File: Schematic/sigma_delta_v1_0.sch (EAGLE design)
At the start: 32 parts, among them IC1 LM340LZ-05, Q1 BS170, Q2 BS170

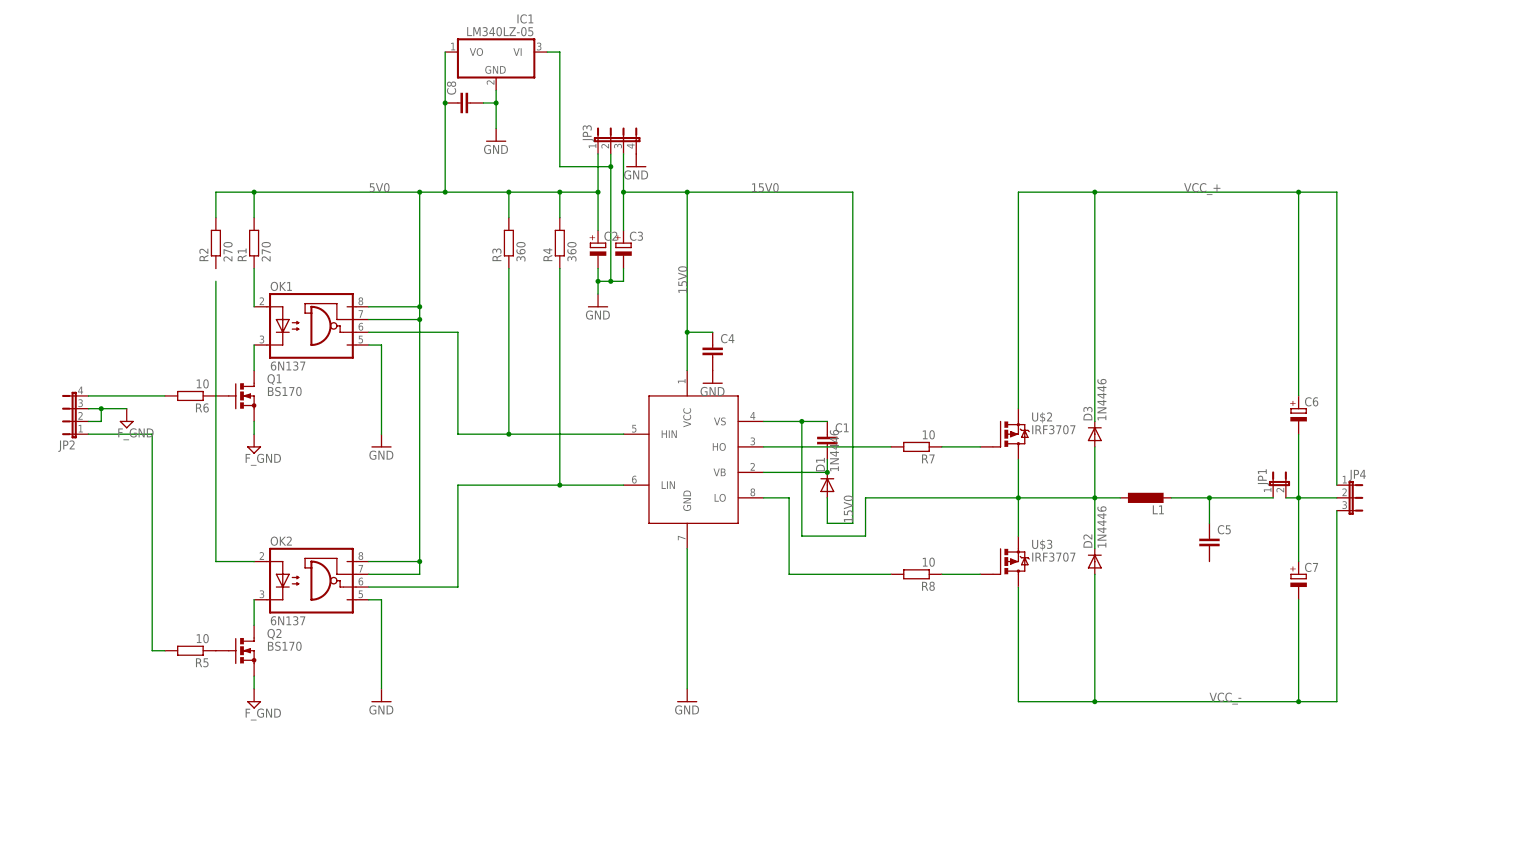
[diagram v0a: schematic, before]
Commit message: started reworking the scematic
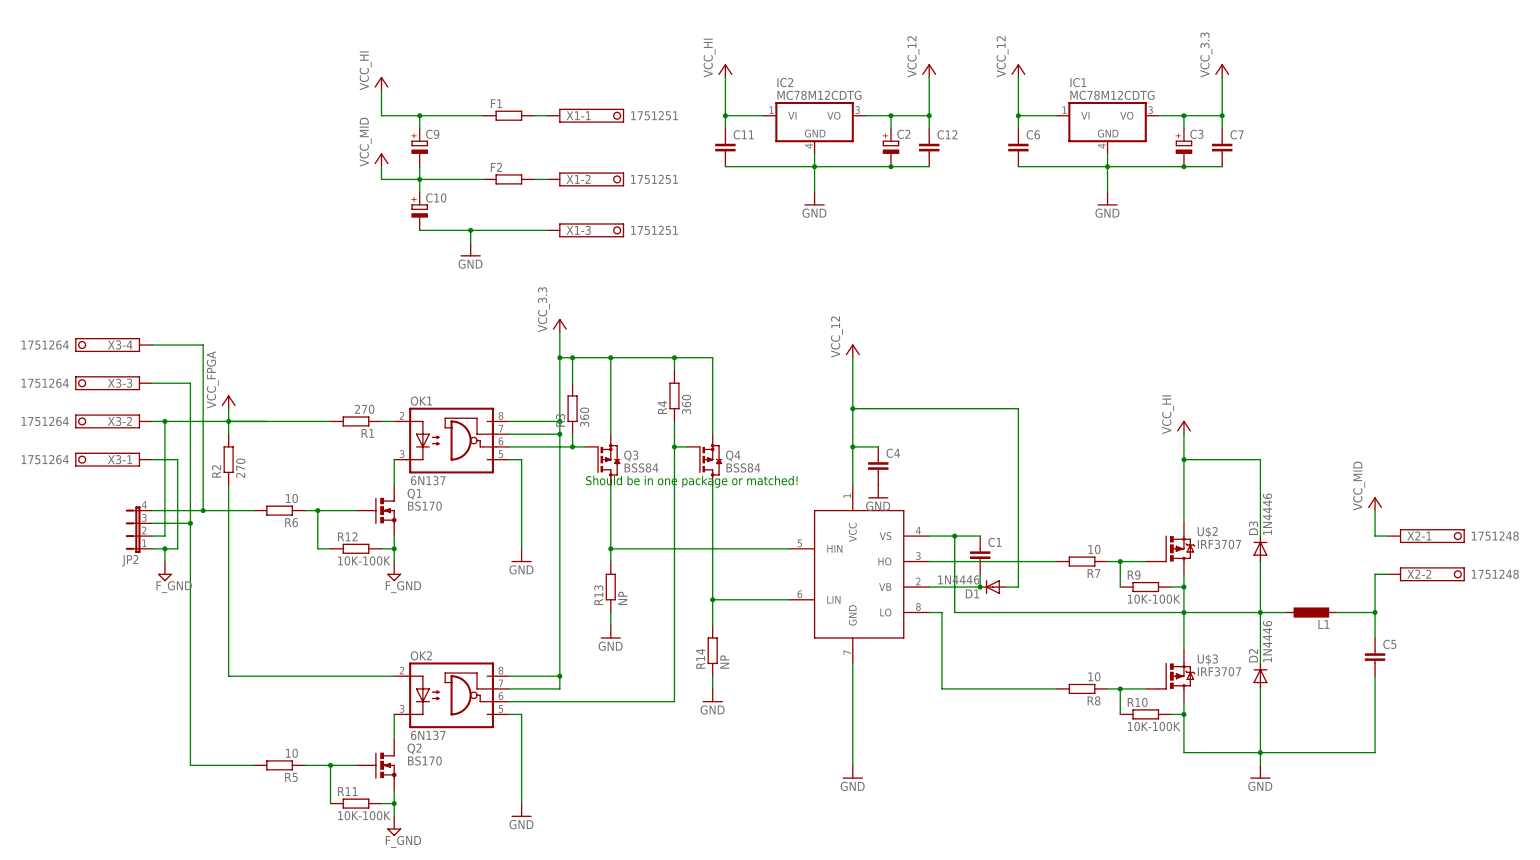
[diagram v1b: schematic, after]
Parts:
- removed C8: (no value), rcl:C-EU025-030X050
- removed JP1: (no value), jumper:JP1E
- removed JP3: (no value), jumper:JP4E
- removed JP4: (no value), jumper:JP2E
- added C10, C9: (no value), rcl:CPOL-EUE2.5-7
- added C11, C12: (no value), rcl:C-EUC0603
- added F1, F2: (no value), rcl:R-EU_M1206
- added IC2: MC78M12CDTG, linear:MC78M12CDTG
- added Q3, Q4: BSS84, transistor-small-signal:BSS84
- added R10, R11, R12, R9: 10K-100K, eagle-ltspice:RR0603
- added R13, R14: NP, eagle-ltspice:RR0603
- added X1: 1751251, con-phoenix-350:1751251
- added X2: 1751248, con-phoenix-350:1751248
- added X3: 1751264, con-phoenix-350:1751264
- C6, C7: device rcl:CPOL-EUE2.5-7 -> rcl:C-EUC0603
- IC1: value LM340LZ-05 -> MC78M12CDTG; device linear:LM340LZ-05 -> linear:MC78M12CDTG
- R1, R2, R3, R4, R5, R6, R7, R8: device eagle-ltspice:R0207/10 -> eagle-ltspice:RR0603
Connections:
- removed net 15V0: C3.+, C4.1, D1.A, JP3.3, U$1.VCC
- removed net 5V0: C2.+, C8.1, IC1.VO, JP3.1, OK1.VCC, OK1.VE, OK2.VCC, OK2.VE, R1.2, R2.2, R3.2, R4.2
- removed net N$8: OK2.VO, R4.1
- removed net VCC_+: C6.+, D3.C, JP4.1, U$2.S
- removed net VCC_-: C7.-, D2.A, JP4.3, U$3.D
- new net N$18: F1.2, X1-1.K
- new net N$20: F2.2, X1-2.K
- new net N$21: Q4.D, R14.2, U$1.LIN
- new net N$22: OK2.VO, Q4.G, R4.1
- new net VCC_12: C12.1, C2.+, C4.1, C6.1, D1.A, IC1.VI, IC2.VO, U$1.VCC
- new net VCC_3.3: C3.+, C7.1, IC1.VO, OK1.VCC, OK1.VE, OK2.VCC, OK2.VE, Q3.S, Q4.S, R3.2, R4.2
- new net VCC_FPGA: JP2.2, R1.2, R2.2, X3-2.K
- new net VCC_HI: C11.1, C9.+, D3.C, F1.1, IC2.VI, U$2.S
- new net VCC_MID: C10.+, C9.-, F2.1, X2-1.K
- net GND: now also C10.-, C11.2, C12.2, C5.2, C6.2, C7.2, D2.A, IC2.GND, JP2.1, R10.2, R11.2, R12.2, R13.1, R14.1, U$3.D, X1-3.K, X3-1.K; no longer C8.2, IC1.VI, JP2.2, JP2.3, JP3.2, JP3.4
- net N$1: now also X3-4.K
- net N$10: now also X2-2.K; no longer JP1.1
- net N$11: now also R11.1
- net N$12: now also R12.1
- net N$14: now also R9.1
- net N$15: now also R10.1
- net N$19: now also Q3.D, R13.2, U$1.HIN; no longer C6.-, C7.+, JP1.2, JP4.2
- net N$2: now also JP2.3, X3-3.K; no longer JP2.1
- net N$6: now also R2.1
- net N$7: now also Q3.G; no longer U$1.HIN
- net N$9: now also R9.2
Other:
- note added: "Should be in one package or matched!"
- moved on the sheet: C1, C2, C3, C4, C5, D1, D2, D3, JP2, L1, OK1, OK2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
